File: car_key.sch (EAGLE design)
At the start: 52 parts, among them IC1 MAX3232ECD, IC2 LM1117MPX-3.3_NOPB, IC3 NRF24L01P-R7, Q1 16M, Q2 BSS816NWH6327XTSA1, SW1 B3U-1000P, SW2 B3U-1000P, U2 ATMEGA328P-AU, X1 RS232, Y1 8MHz

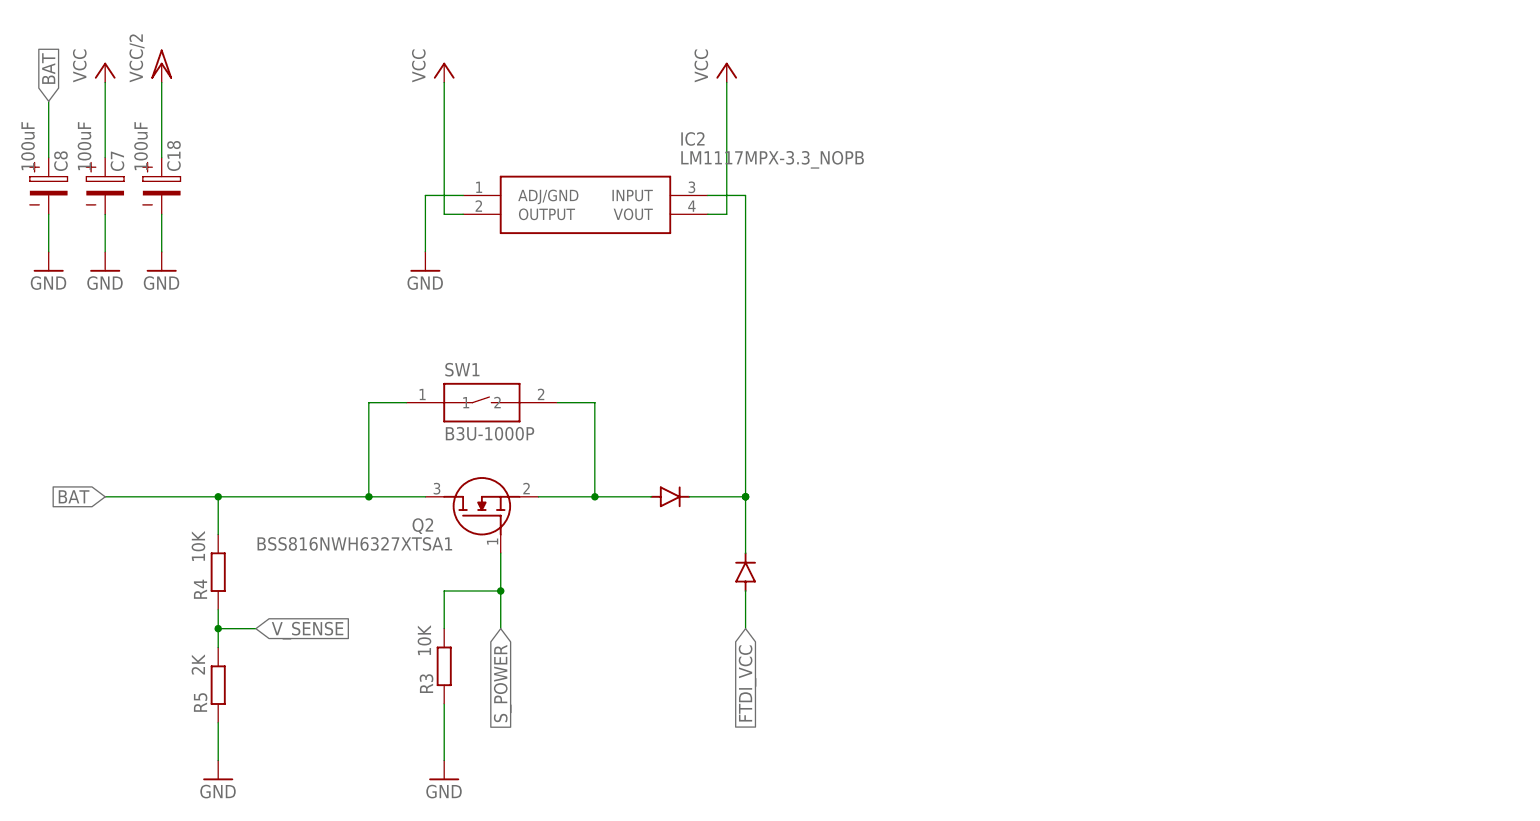
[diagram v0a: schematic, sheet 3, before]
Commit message: changes
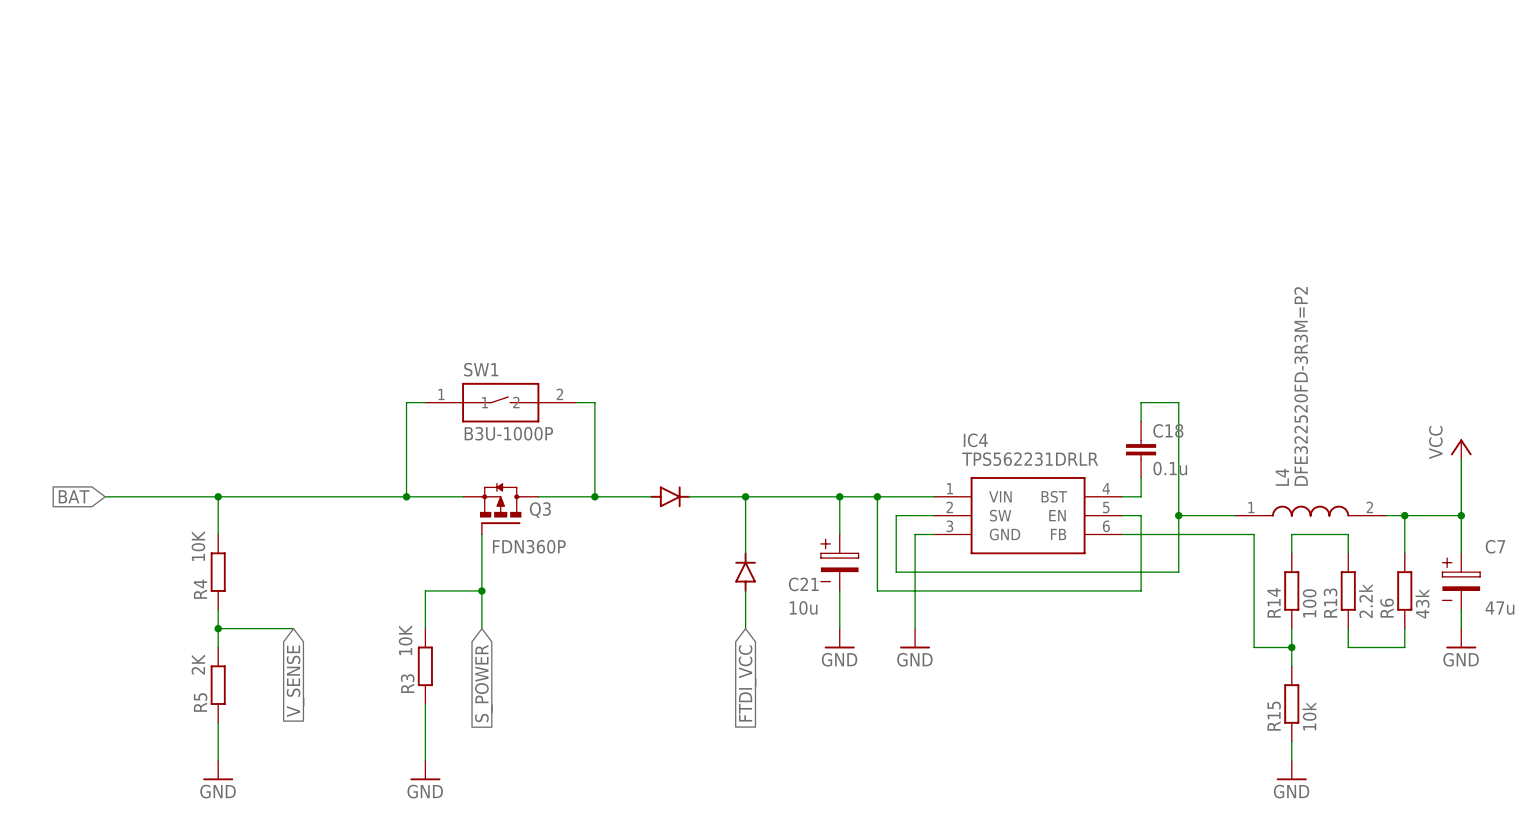
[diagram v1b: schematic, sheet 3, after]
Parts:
- removed C8: 100uF, Wurth_Elektronik_Passive_Capacitors_rev18b:WCAP-ASLI_6,3X7,7_865080445010
- removed IC2: LM1117MPX-3.3_NOPB, LM1117MPX-3.3_NOPB:LM1117MPX-3.3_NOPB
- removed Q2: BSS816NWH6327XTSA1, BSS816NWH6327XTSA1:BSS816NWH6327XTSA1
- added C21: 10u, Wurth_Elektronik_Passive_Capacitors_rev18b:WCAP-ASLI_4X5,5_865080340001
- added IC4: TPS562231DRLR, TPS562231DRLR:TPS562231DRLR
- added L4: DFE322520FD-3R3M=P2, DFE322520FD-3R3M=P2:DFE322520FD-3R3M=P2
- added Q3: FDN360P, transistor-power:FDN360P
- added R13: 2.2k, rcl:R-EU_R0805
- added R14: 100, rcl:R-EU_R0805
- added R15: 10k, rcl:R-EU_R0805
- added R6: 43k, rcl:R-EU_R0805
- C18: value 100uF -> 0.1u; device Wurth_Elektronik_Passive_Capacitors_rev18b:WCAP-ASLI_6,3X7,7_865080445010 -> rcl:C-EUC0805
- C7: value 100uF -> 47u; device Wurth_Elektronik_Passive_Capacitors_rev18b:WCAP-ASLI_6,3X7,7_865080445010 -> Wurth_Elektronik_Passive_Capacitors_rev18b:WCAP-ASLI_4X5,5_865080140004
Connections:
- removed net VCC/2: C18.1
- new net N$24: C18.1, IC4.SW, L4.1
- new net N$25: C18.2, IC4.BST
- new net N$26: R13.2, R14.2
- new net N$30: R13.1, R6.1
- new net N$31: IC4.FB, R14.1, R15.2
- net BAT: now also Q3.S; no longer C8.1, Q2.D
- net GND: now also C21.2, IC4.GND, R15.1; no longer C18.2, C8.2, IC2.ADJ/GND
- net N$27: now also C21.1, IC4.EN, IC4.VIN; no longer IC2.INPUT
- net N$33: now also Q3.D; no longer Q2.S
- net S_POWER: now also Q3.G; no longer Q2.G
- net VCC: now also L4.2, R6.2; no longer IC2.OUTPUT, IC2.VOUT
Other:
- moved on the sheet: C7, FTDI-1, FTDI-2, FTDI-3, FTDI-4, FTDI-5, FTDI-6, R3, SW1
